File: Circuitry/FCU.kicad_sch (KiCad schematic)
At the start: 30 parts, among them J1 Conn_01x04_Pin, J2 USB_C_Receptacle_USB2.0_16P, J3 Conn_01x06_Pin, J4 Conn_01x04_Pin, J5 Conn_01x04_Pin, J6 Conn_01x09_Pin, SW1 SW_SPDT, SW2 SW_Push, U1 STM32F405RGTx, U2 AMS1117-3.3, Y1 8MHz

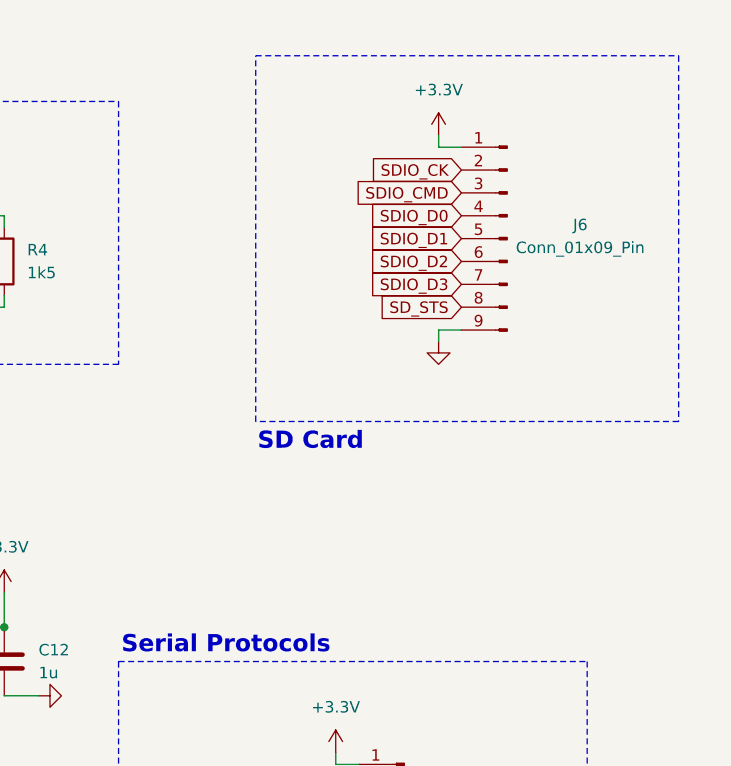
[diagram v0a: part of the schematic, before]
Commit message: added some readme notes
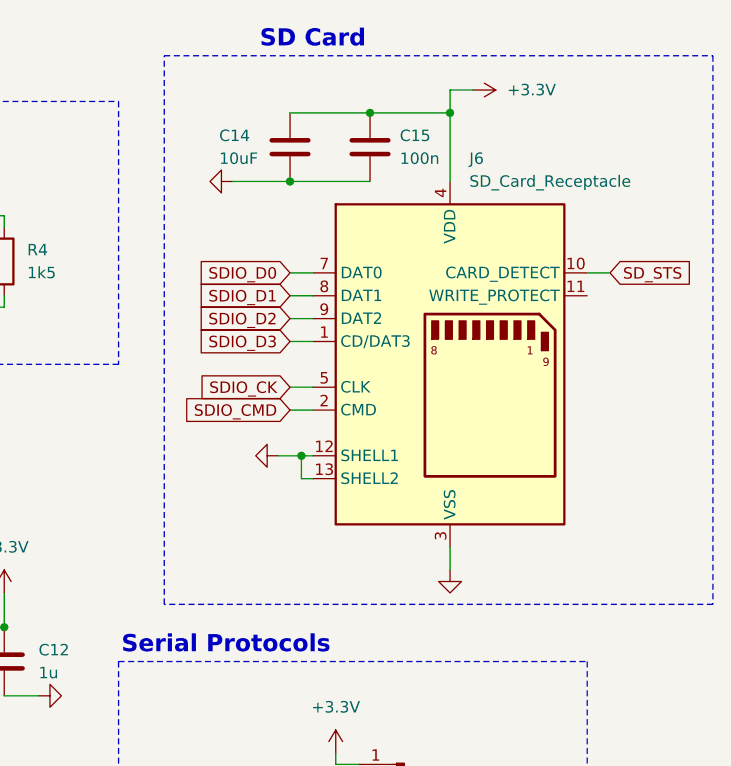
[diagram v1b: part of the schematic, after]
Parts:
- removed J6: Conn_01x09_Pin, Connector_JST:JST_PH_S9B-PH-K_1x09_P2.00mm_Horizontal, symbol Connector:Conn_01x09_Pin
- added C14: 10uF, Capacitor_SMD:C_1206_3216Metric, symbol Device:C
- added C15: 100n, Capacitor_SMD:C_0603_1608Metric, symbol Device:C
- added J6: SD_Card_Receptacle, Connector_Card:SD_Hirose_DM1AA_SF_PEJ82, symbol Connector:SD_Card_Receptacle
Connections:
- net +3.3V: now also C14.1, C15.1, J6.4 (VDD)
- net GND: now also C14.2, C15.2, J6.12 (SHELL1), J6.13 (SHELL2), J6.3 (VSS), J6.6 (VSS)
- net SDIO_CK: now also J6.5 (CLK)
- net SDIO_CMD: now also J6.2 (CMD)
- net SDIO_D0: now also J6.7 (DAT0)
- net SDIO_D1: now also J6.8 (DAT1)
- net SDIO_D2: now also J6.9 (DAT2)
- net SDIO_D3: now also J6.1 (CD/DAT3)
- net SD_STS: now also J6.10 (CARD_DETECT)
